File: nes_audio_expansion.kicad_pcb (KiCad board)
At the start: 2 copper layers, 19.7 x 5.7 mm, 4 parts, among them J1 Expansion_Port, J2 NESRGB

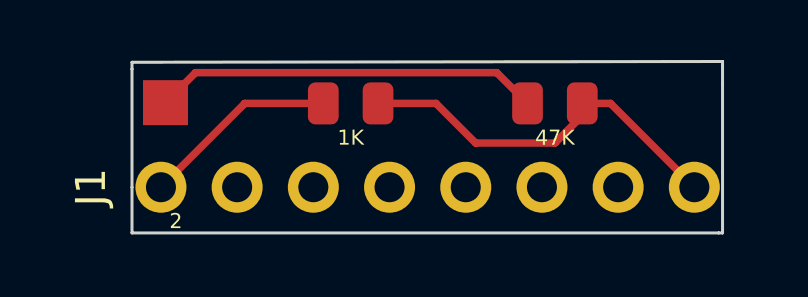
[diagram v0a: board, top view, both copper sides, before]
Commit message: Add files via upload
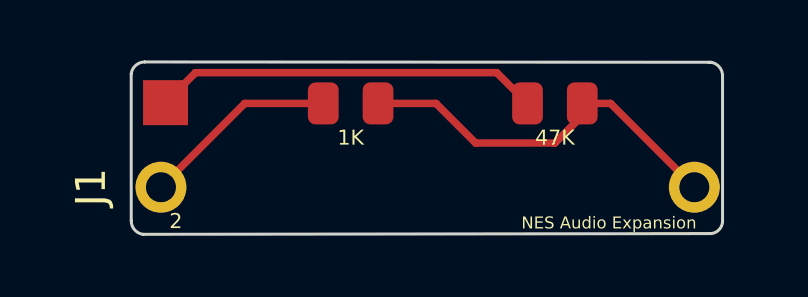
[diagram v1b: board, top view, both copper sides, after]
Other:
- outline, holes or cut-outs redrawn
- board text added: "NES Audio Expansion"
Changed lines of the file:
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@@
     (pad "1" thru_hole circle (at 0 0 90) (size 1.7 1.7) (drill 1) (layers "*.Cu" "*.Mask")
       (net 1 "Net-(J1-2)") (pinfunction "2") (pintype "passive"))
-    (pad "2" thru_hole oval (at 0 2.54 90) (size 1.7 1.7) (drill 1) (layers "*.Cu" "*.Mask")
+    (pad "2" thru_hole oval (at 0 2.54 90) (size 0.1 0.1) (drill 1) (layers "*.Cu" "*.Mask")
       (net 2 "unconnected-(J1-3-Pad2)") (pinfunction "3") (pintype "passive+no_connect"))
-    (pad "3" thru_hole oval (at 0 5.08 90) (size 1.7 1.7) (drill 1) (layers "*.Cu" "*.Mask")
+    (pad "3" thru_hole oval (at 0 5.08 90) (size 0.1 0.1) (drill 1) (layers "*.Cu" "*.Mask")
       (net 3 "unconnected-(J1-4-Pad3)") (pinfunction "4") (pintype "passive+no_connect"))
-    (pad "4" thru_hole oval (at 0 7.62 90) (size 1.7 1.7) (drill 1) (layers "*.Cu" "*.Mask")
+    (pad "4" thru_hole oval (at 0 7.62 90) (size 0.1 0.1) (drill 1) (layers "*.Cu" "*.Mask")
       (net 4 "unconnected-(J1-5-Pad4)") (pinfunction "5") (pintype "passive+no_connect"))
-    (pad "5" thru_hole oval (at 0 10.16 90) (size 1.7 1.7) (drill 1) (layers "*.Cu" "*.Mask")
+    (pad "5" thru_hole oval (at 0 10.16 90) (size 0.1 0.1) (drill 1) (layers "*.Cu" "*.Mask")
       (net 5 "unconnected-(J1-6-Pad5)") (pinfunction "6") (pintype "passive+no_connect"))
-    (pad "6" thru_hole oval (at 0 12.7 90) (size 1.7 1.7) (drill 1) (layers "*.Cu" "*.Mask")
+    (pad "6" thru_hole oval (at 0 12.7 90) (size 0.1 0.1) (drill 1) (layers "*.Cu" "*.Mask")
       (net 6 "unconnected-(J1-7-Pad6)") (pinfunction "7") (pintype "passive+no_connect"))
-    (pad "7" thru_hole oval (at 0 15.24 90) (size 1.7 1.7) (drill 1) (layers "*.Cu" "*.Mask")
+    (pad "7" thru_hole oval (at 0 15.24 90) (size 0.1 0.1) (drill 1) (layers "*.Cu" "*.Mask")
       (net 7 "unconnected-(J1-8-Pad7)") (pinfunction "8") (pintype "passive+no_connect"))
     (pad "8" thru_hole oval (at 0 17.78 90) (size 1.7 1.7) (drill 1) (layers "*.Cu" "*.Mask")
@@
       (net 9 "Net-(J2-Pin_1)") (pinfunction "Pin_1") (pintype "passive"))
   )
-  (gr_line (start 128.651 115.824) (end 148.209 115.824)
+  (gr_arc (start 129.018142 115.870205) (mid 128.737407 115.717158) (end 128.6256 115.4176)
     (stroke (width 0.1) (type default)) (layer "Edge.Cuts"))
-  (gr_line (start 148.336 115.824) (end 148.209 115.824)
+  (gr_arc (start 128.624953 110.516736) (mid 128.778 110.236) (end 129.077558 110.124194)
     (stroke (width 0.1) (type default)) (layer "Edge.Cuts"))
-  (gr_line (start 148.336 110.8456) (end 148.336 110.236)
+  (gr_line (start 147.8788 110.1344) (end 129.077558 110.124194)
     (stroke (width 0.1) (type default)) (layer "Edge.Cuts"))
-  (gr_line (start 148.336 110.109) (end 148.336 110.236)
+  (gr_arc (start 147.943458 110.133753) (mid 148.224193 110.2868) (end 148.336 110.586358)
     (stroke (width 0.1) (type default)) (layer "Edge.Cuts"))
-  (gr_line (start 128.651 110.363) (end 128.651 110.1344)
+  (gr_arc (start 148.336 115.452873) (mid 148.212985 115.7224) (end 147.943458 115.845415)
     (stroke (width 0.1) (type default)) (layer "Edge.Cuts"))
-  (gr_line (start 128.651 114.3) (end 128.651 110.363)
+  (gr_line (start 148.336 115.452873) (end 148.336 110.8456)
     (stroke (width 0.1) (type default)) (layer "Edge.Cuts"))
-  (gr_line (start 128.651 114.3) (end 128.651 115.824)
+  (gr_line (start 147.8788 110.1344) (end 147.943458 110.133753)
     (stroke (width 0.1) (type default)) (layer "Edge.Cuts"))
-  (gr_line (start 128.651 110.1344) (end 148.336 110.109)
+  (gr_line (start 148.336 110.8456) (end 148.336 110.586358)
     (stroke (width 0.1) (type default)) (layer "Edge.Cuts"))
-  (gr_line (start 148.336 113.792) (end 148.336 115.824)
+  (gr_line (start 147.943458 115.845415) (end 129.018142 115.870205)
     (stroke (width 0.1) (type default)) (layer "Edge.Cuts"))
-  (gr_line (start 148.336 113.792) (end 148.336 110.8456)
+  (gr_line (start 128.624953 110.516736) (end 128.6256 115.4176)
     (stroke (width 0.1) (type default)) (layer "Edge.Cuts"))
+  (gr_text "NES Audio Expansion" (at 141.6304 115.7224) (layer "F.SilkS")
+    (effects (font (size 0.4 0.4) (thickness 0.06)) (justify left bottom))
+  )
   (gr_text "2" (at 129.8956 115.7224) (layer "F.SilkS")
     (effects (font (size 0.5 0.5) (thickness 0.06)) (justify left bottom))
